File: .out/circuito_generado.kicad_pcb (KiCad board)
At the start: 2 copper layers, 150 x 100 mm, 7 parts, among them U1 DIP-8_W7.62mm

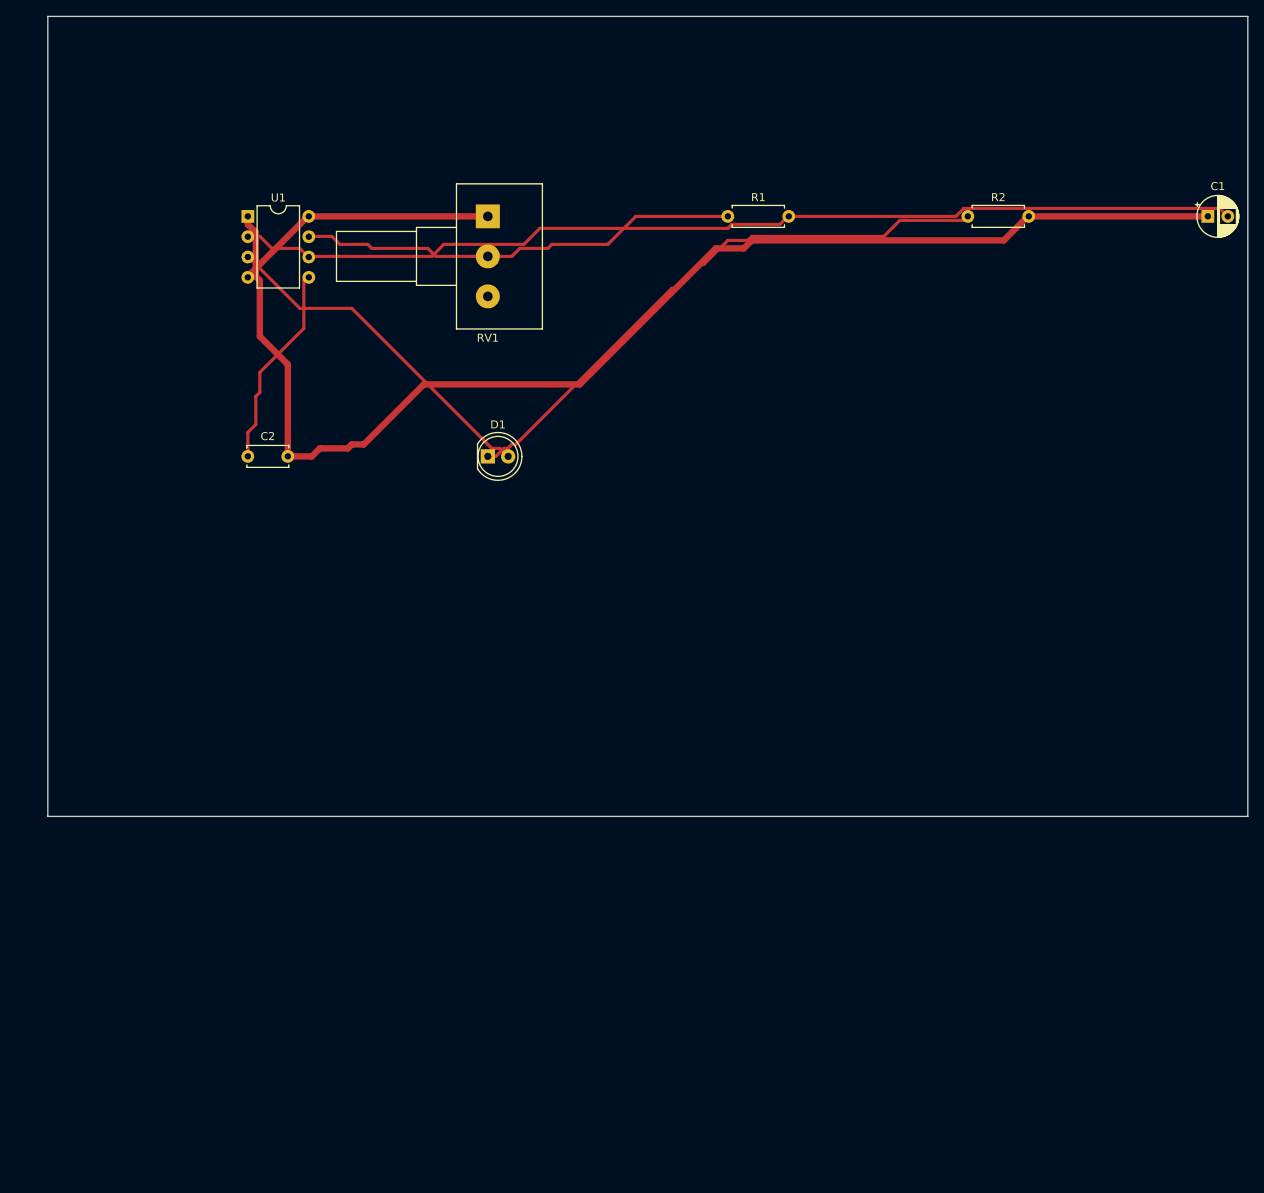
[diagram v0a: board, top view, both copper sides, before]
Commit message: Version v1.0.18
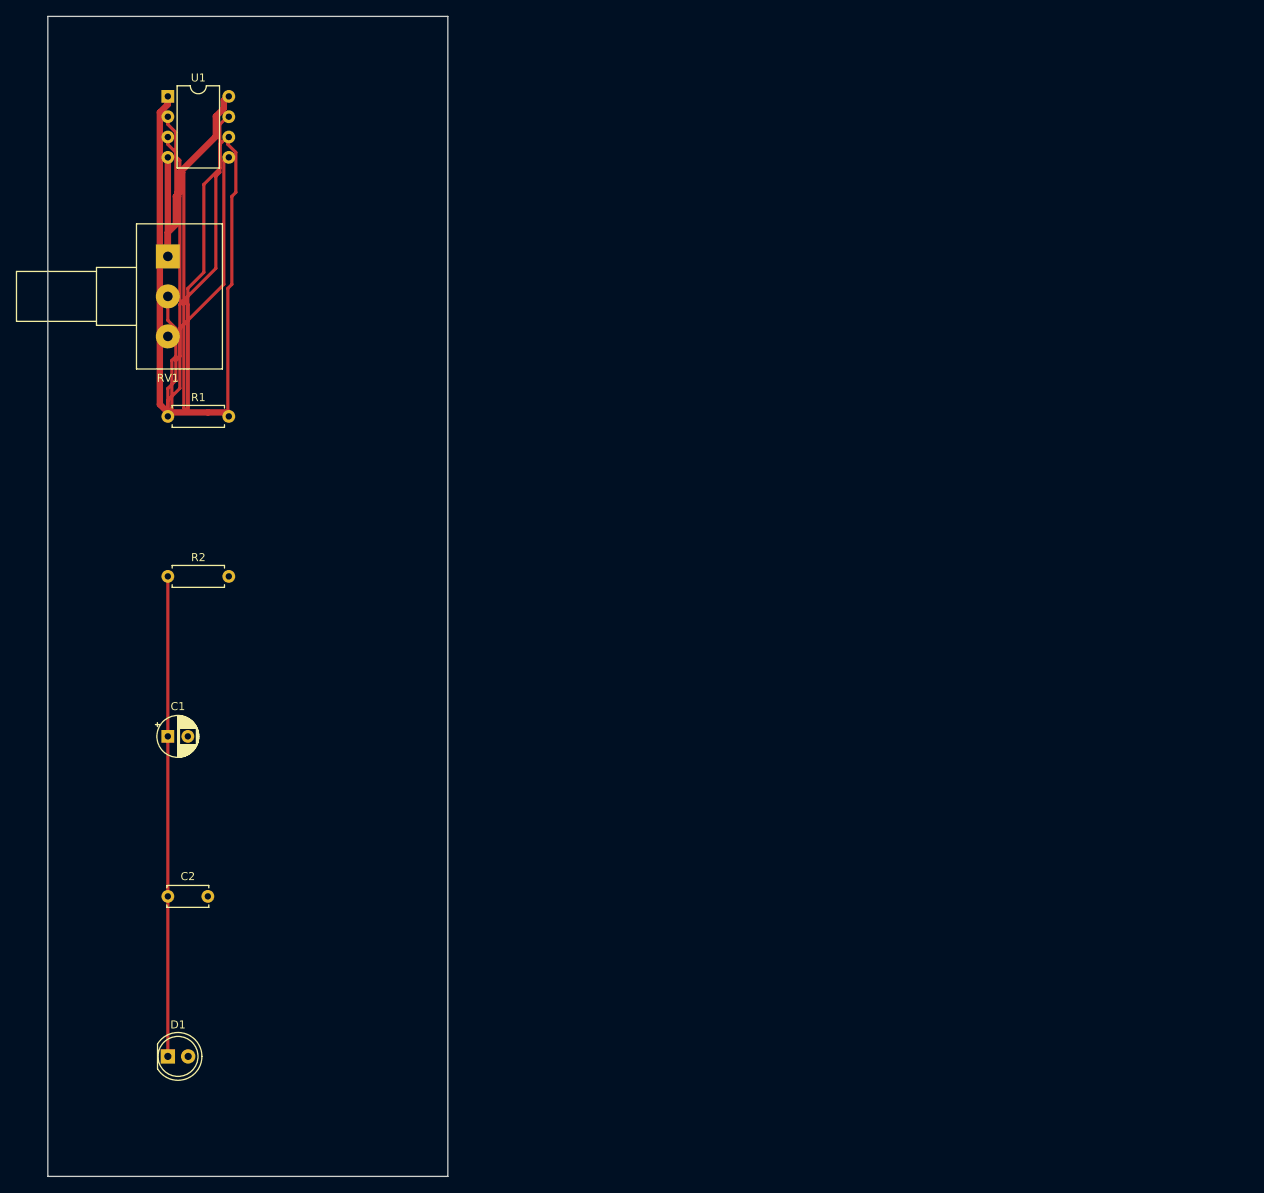
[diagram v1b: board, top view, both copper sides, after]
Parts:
- moved C1 145.3 mm to (15.0, 90.0)
- moved R2 109.7 mm to (15.0, 70.0)
- moved D1 85.0 mm to (15.0, 130.0)
- moved R1 74.3 mm to (15.0, 50.0)
- moved C2 55.9 mm to (15.0, 110.0)
- moved RV1 40.3 mm to (15.0, 30.0)
- moved U1 18.0 mm to (15.0, 10.0)
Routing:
- net GND: track 159.5 -> 47.8 mm
- net NET_RB_TRIGGER_THRESHOLD: track 126.4 -> 109.9 mm
- net NET_LED_CURRENT_LIMIT: track 72.4 -> 60.0 mm
- net NET_CONTROL_VOLTAGE: track 25.6 -> 35.1 mm
- net NET_LED_OUT: track 42.9 -> 35.5 mm
- net VCC_9V: track 33.1 -> 35.6 mm
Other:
- board size 150 x 100 mm -> 50 x 145 mm
